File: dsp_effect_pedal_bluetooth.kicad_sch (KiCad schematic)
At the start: 5 parts, among them J1 USB_C_Receptacle_PowerOnly_24P

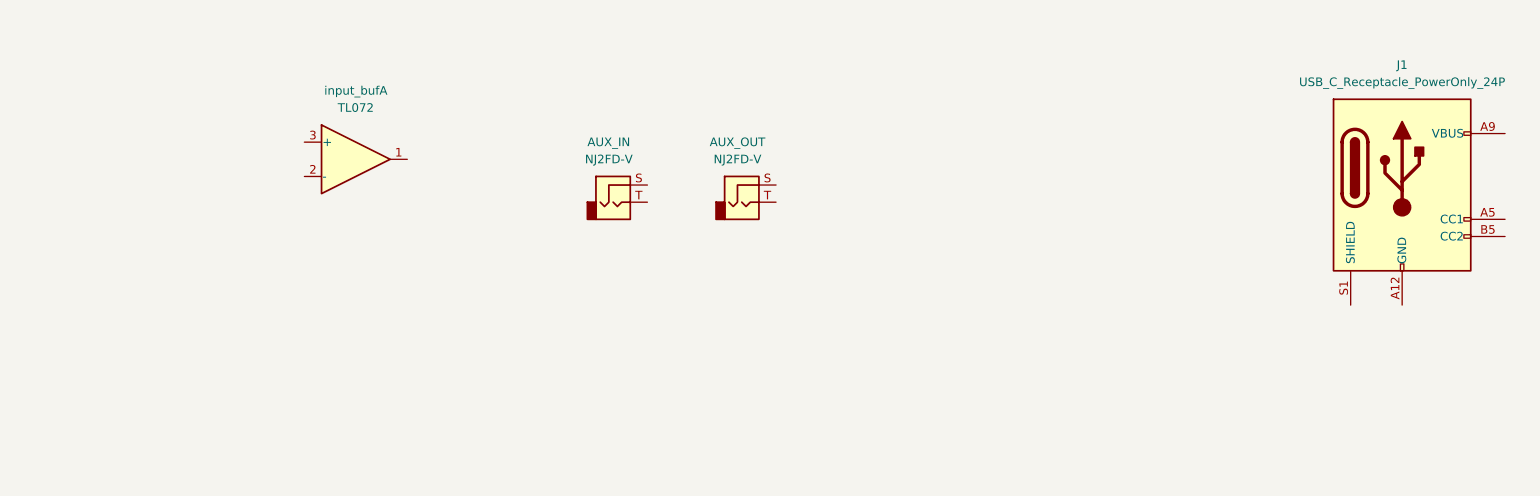
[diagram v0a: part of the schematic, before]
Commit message: input buffer
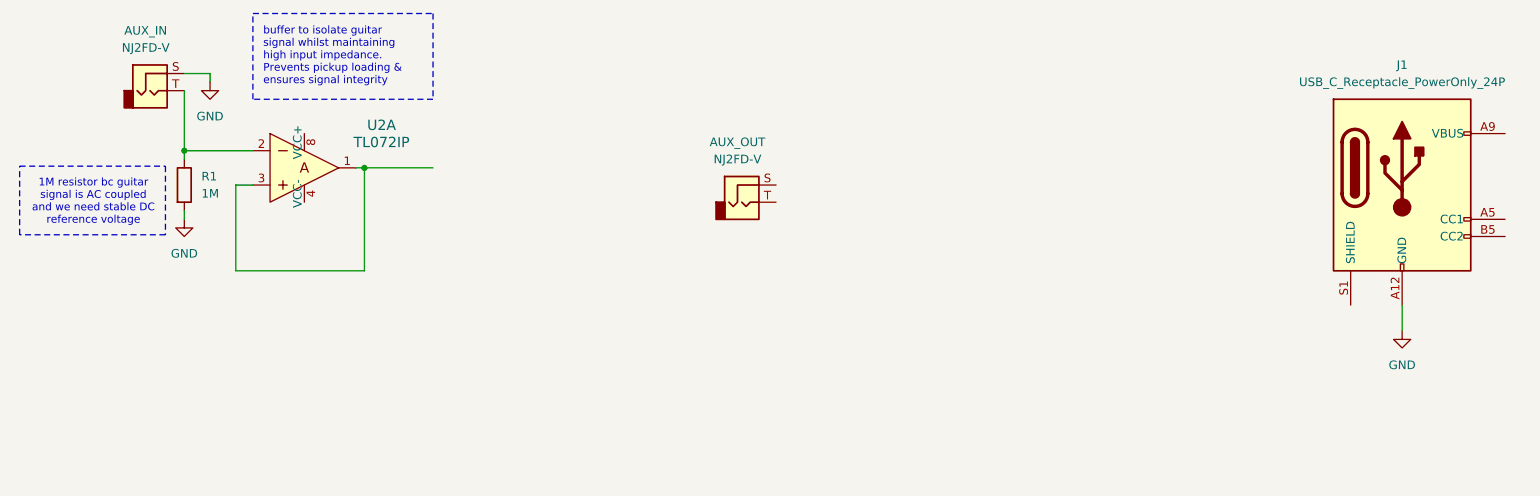
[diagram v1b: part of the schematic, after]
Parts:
- removed input_buf: TL072, symbol Amplifier_Operational:TL072
- added R1: 1M, symbol Device:R
- added U2: TL072IP, digikey-footprints:DIP-8_W7.62mm, symbol dk_Linear-Amplifiers-Instrumentation-OP-Amps-Buffer-Amps:TL072IP
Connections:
- net GND: now reaches J1.A1 (GND), J1.A12 (GND), J1.B1 (GND), J1.B12 (GND)
- net GND: now also AUX_IN.S, R1.2
- net at AUX_IN.T: now also R1.1, U2.2
- new net: U2.1, U2.3
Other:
- note added: "1M resistor bc guitar signal is AC coupled and we need stable DC reference voltage"
- note added: "buffer to isolate guitar signal whilst maintaining high input impedance. Prevents pickup loading & ensures signal integrity"
- moved on the sheet: AUX_IN

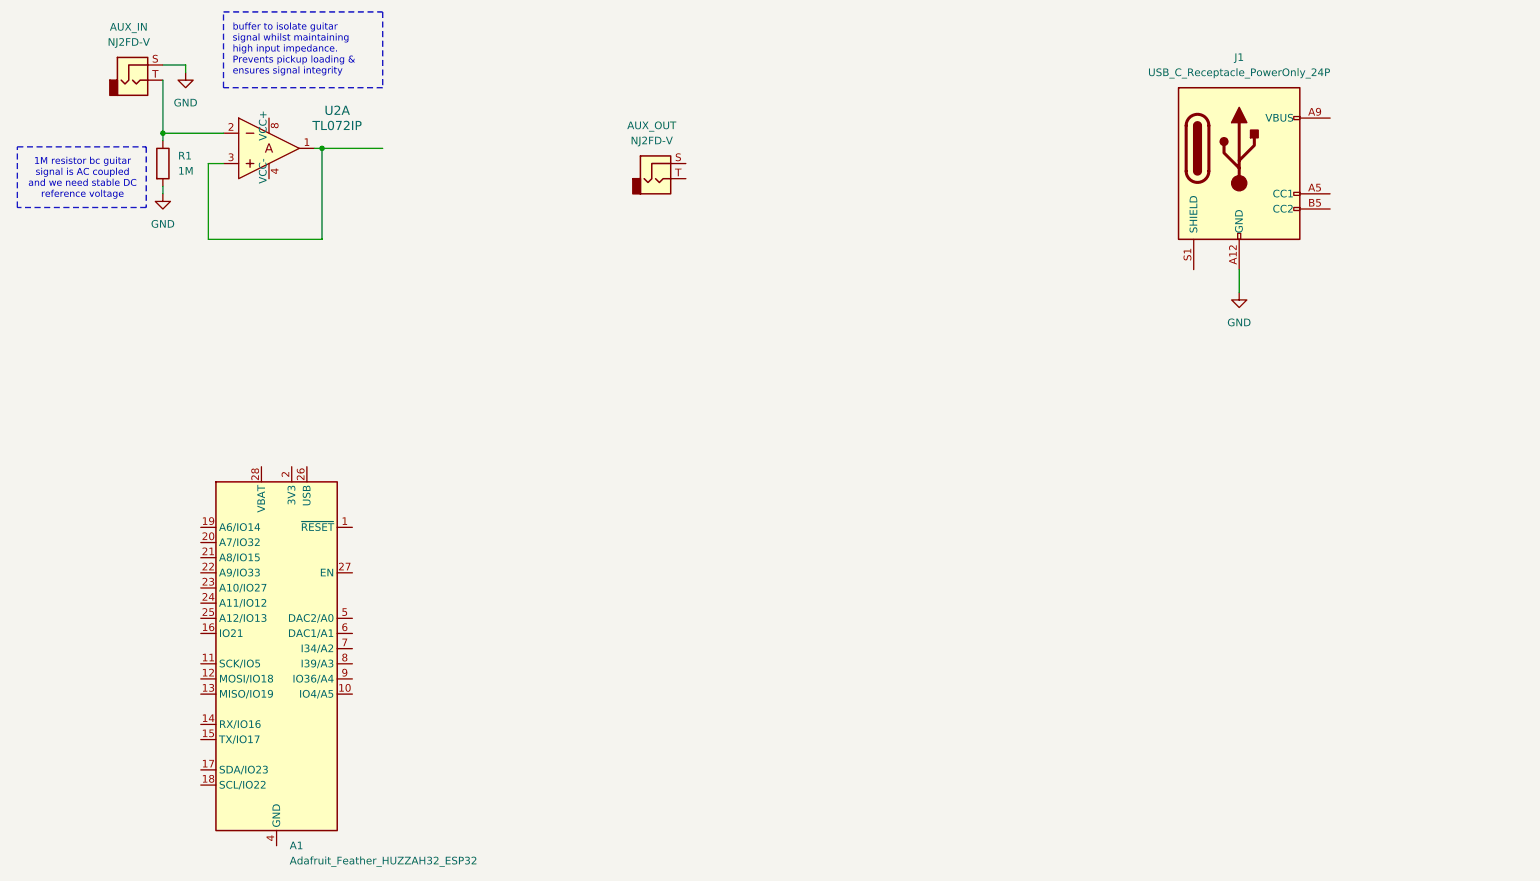
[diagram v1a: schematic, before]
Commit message: step up converter work
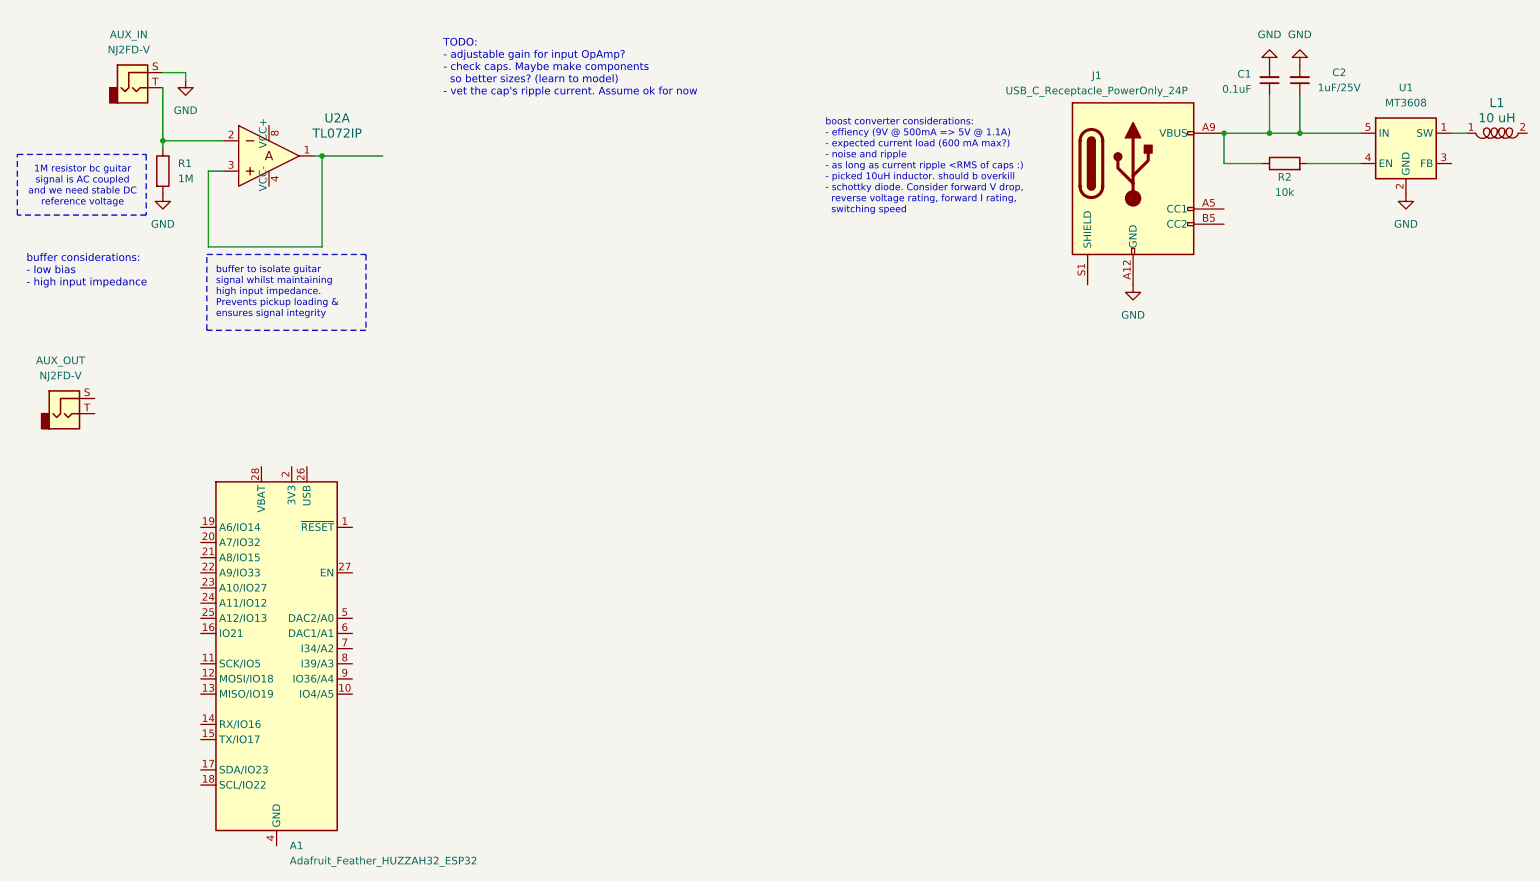
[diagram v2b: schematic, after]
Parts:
- added 1uF/25V: 1uF_0603_25V, 4ms_Capacitor:C_0603, symbol PCM_4ms_Capacitor:1uF_0603_25V
- added C1: 0.1uF_0603_16V, 4ms_Capacitor:C_0603, symbol PCM_4ms_Capacitor:0.1uF_0603_16V
- added L1: 10 uH, digikey-footprints:1206, symbol dk_Fixed-Inductors:82103C
- added R2: 10k_0603, 4ms_Resistor:R_0603, symbol PCM_4ms_Resistor:10k_0603
- added U1: MT3608, Package_TO_SOT_SMD:SOT-23-6, symbol Regulator_Switching:MT3608
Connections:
- net GND: now also 1uF/25V.2, C1.2, U1.2 (GND)
- net at J1.A4 (VBUS), J1.A9 (VBUS), J1.B4 (VBUS)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: now also 1uF/25V.1, C1.1, R2.1, U1.5 (IN)
- new net: L1.1, U1.1 (SW)
- new net: R2.2, U1.4 (EN)
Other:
- note added: "TODO: - adjustable gain for input OpAmp? - check caps. Maybe make components so better sizes? (learn to model) - vet the cap's ripple current. Assume ok for now"
- note added: "boost converter considerations: - effiency (9V @ 500mA => 5V @ 1.1A) - expected current load (600 mA max?) - noise and ripple - as long as current ripple <RMS of caps :) - picked 10uH inductor. should b overkill - schottky diode. Consider forward V drop, reverse voltage rating, forward I rating, switching speed"
- note added: "buffer considerations: - low bias - high input impedance"
- moved on the sheet: AUX_IN, AUX_OUT, J1, R1, U2A
